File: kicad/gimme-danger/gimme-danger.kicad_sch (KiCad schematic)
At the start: 54 parts, among them J2 Barrel_Jack, J3 Screw_Terminal_01x06, Q1 AO3400A, Q2 AO3400A, U1 ESP32-S3-WROOM-1, U2 TPD6S300RUKR, U3 U261-241N-4BS2SS, U4 AO4407A, U5 SKRKAEE020, U6 DDTC143EUA, U7 SKRKAEE020, U8 TPS54302

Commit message: Initial partial routing
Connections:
- net VOUT: now also C10.1, U4.5 (D), U4.6 (D), U4.7 (D), U4.8 (D)
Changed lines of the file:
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@@
+    (stroke (width 0) (type default))
+  )
+  (wire (pts (xy 249.682 30.988) (xy 249.682 33.528))
     (stroke (width 0) (type default))
   )
@@
     (stroke (width 0) (type default))
   )
-  (wire (pts (xy 249.682 30.988) (xy 249.682 28.448))
+  (wire (pts (xy 249.682 28.448) (xy 249.682 30.988))
     (stroke (width 0) (type default))
   )
@@
     (stroke (width 0) (type default))
   )
-  (wire (pts (xy 249.682 33.528) (xy 249.682 30.988))
-    (stroke (width 0) (type default))
-  )
   (wire (pts (xy 140.335 64.77) (xy 140.335 69.85))
     (stroke (width 0) (type default))
@@
     (stroke (width 0) (type default))
   )
-  (wire (pts (xy 249.936 30.988) (xy 252.476 30.988))
-    (stroke (width 0) (type default))
-  )
   (wire (pts (xy 234.442 33.528) (xy 234.442 30.988))
     (stroke (width 0) (type default))
@@
     (stroke (width 0) (type default))
   )
+  (wire (pts (xy 249.682 30.988) (xy 252.476 30.988))
+    (stroke (width 0) (type default))
+  )

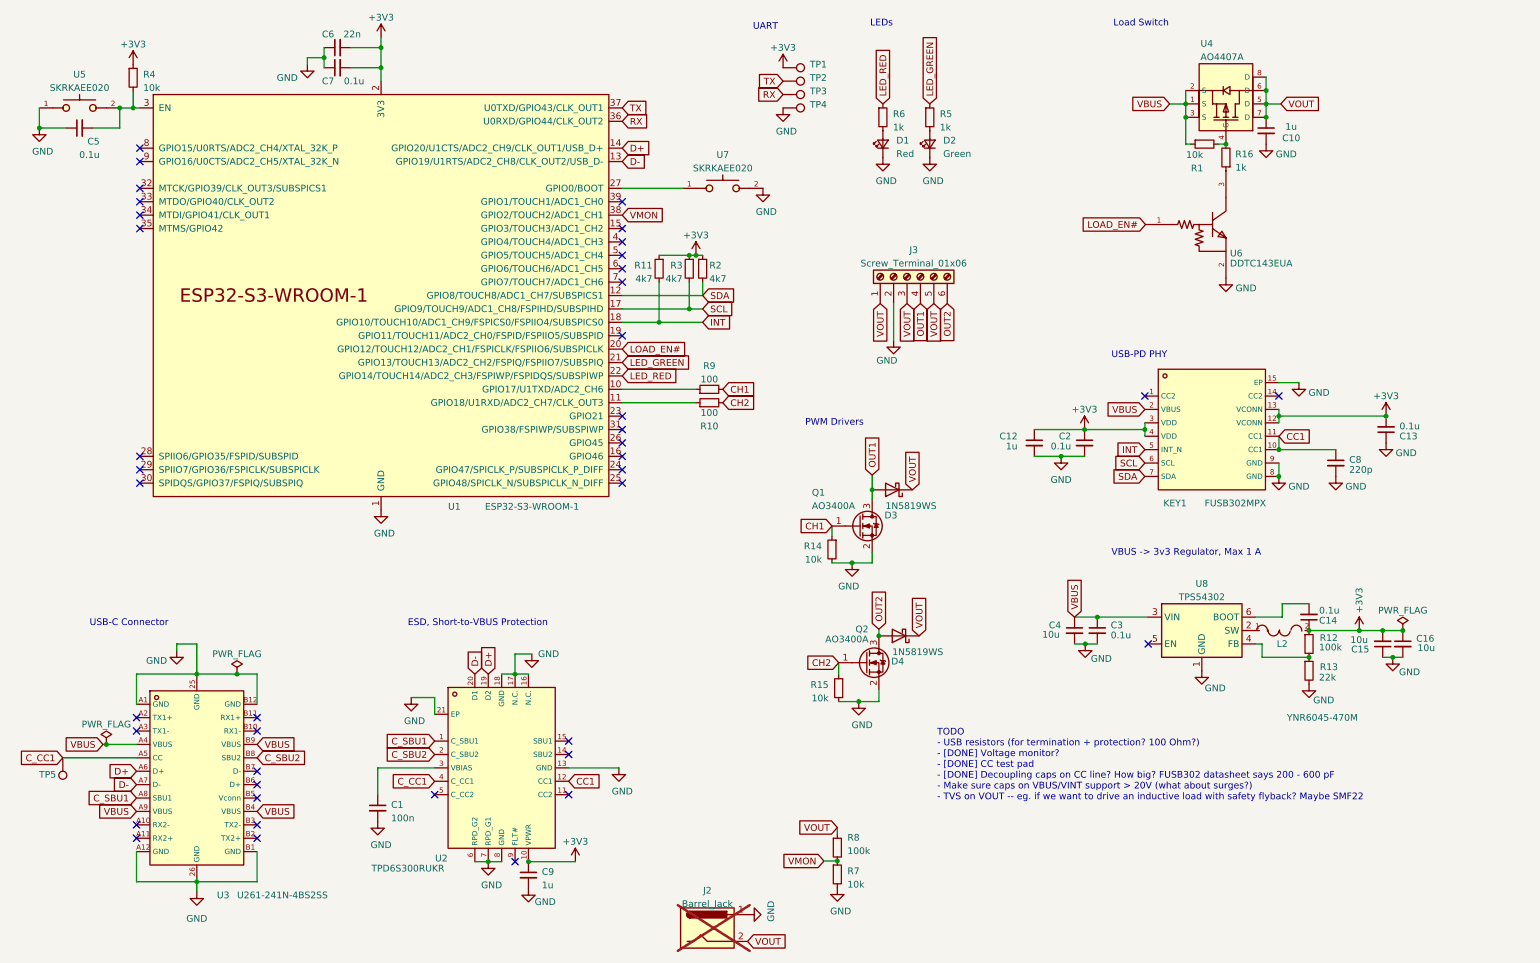
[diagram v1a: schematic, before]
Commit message: Initial routing
Many issues :|
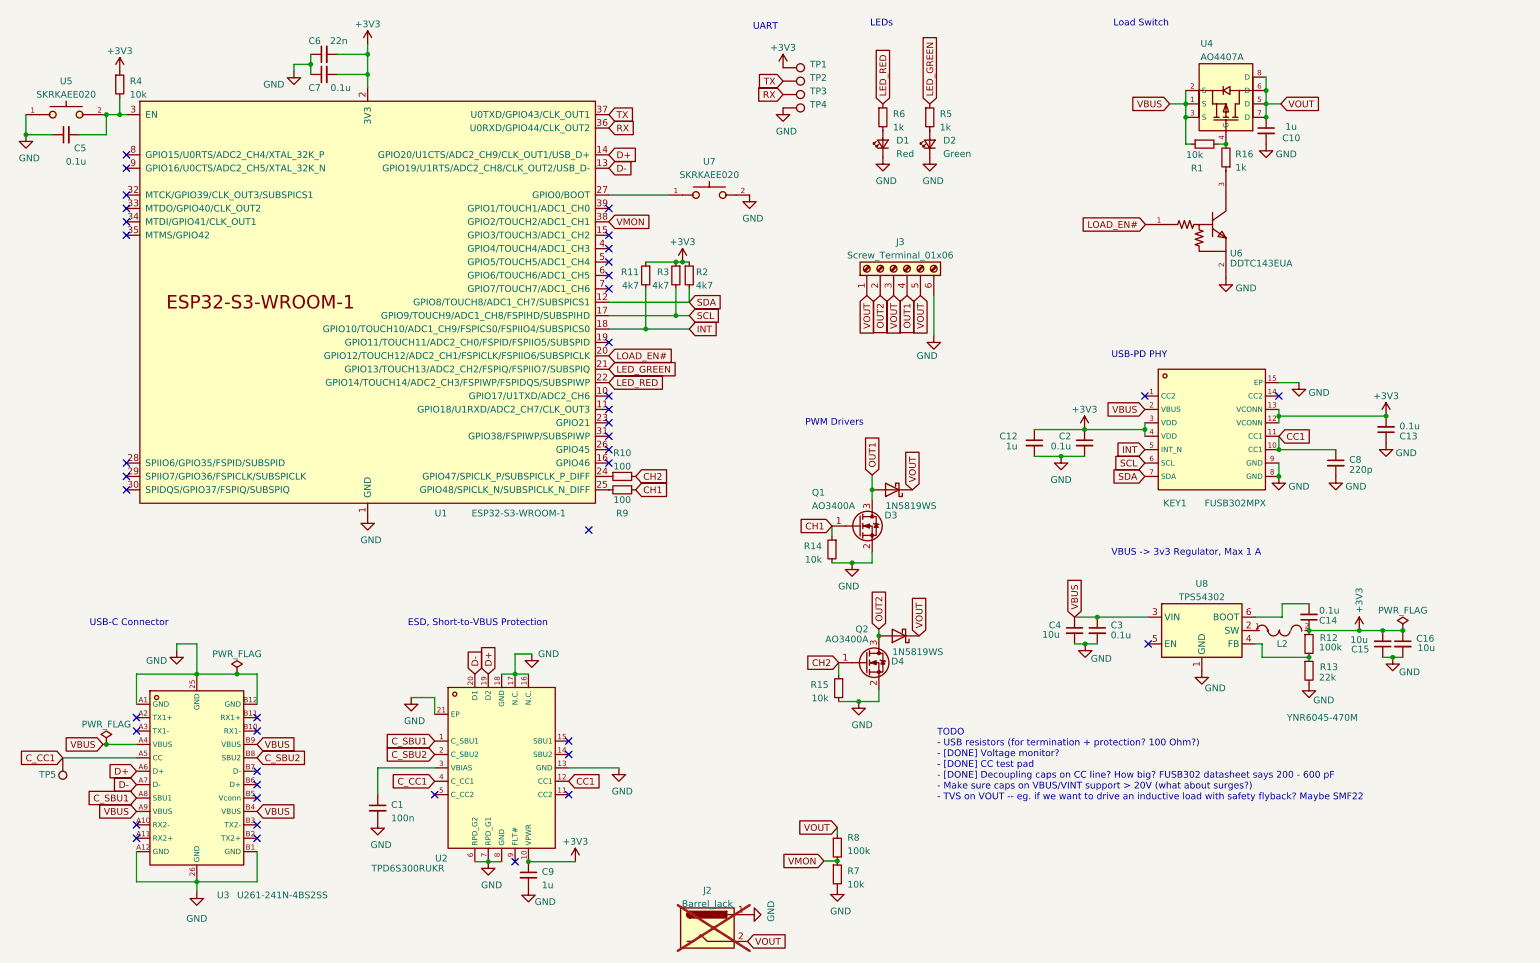
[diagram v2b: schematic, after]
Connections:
- net CH1: now also R9.1; no longer R9.2
- net GND: now also J3.6 (Pin_6); no longer J3.2 (Pin_2)
- net OUT2: now also J3.2 (Pin_2); no longer J3.6 (Pin_6)
- net at U1.10 (GPIO17/U1TXD/ADC2_CH6): no longer R9.1
- net at U1.11 (GPIO18/U1RXD/ADC2_CH7/CLK_OUT3): no longer R10.1
- net at U1.24 (GPIO47/SPICLK_P/SUBSPICLK_P_DIFF): now also R10.1
- net at U1.25 (GPIO48/SPICLK_N/SUBSPICLK_N_DIFF): now also R9.2
- no-connect marks 41 -> 42
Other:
- moved on the sheet: C5, C6, C7, J3, R10, R11, R2, R3, R4, R9, U1, U5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
